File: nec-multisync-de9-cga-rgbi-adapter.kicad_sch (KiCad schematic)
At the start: 8 parts, among them J1 DE9_Plug, J2 DE15_Receptacle_HighDensity, J3 DIN-8

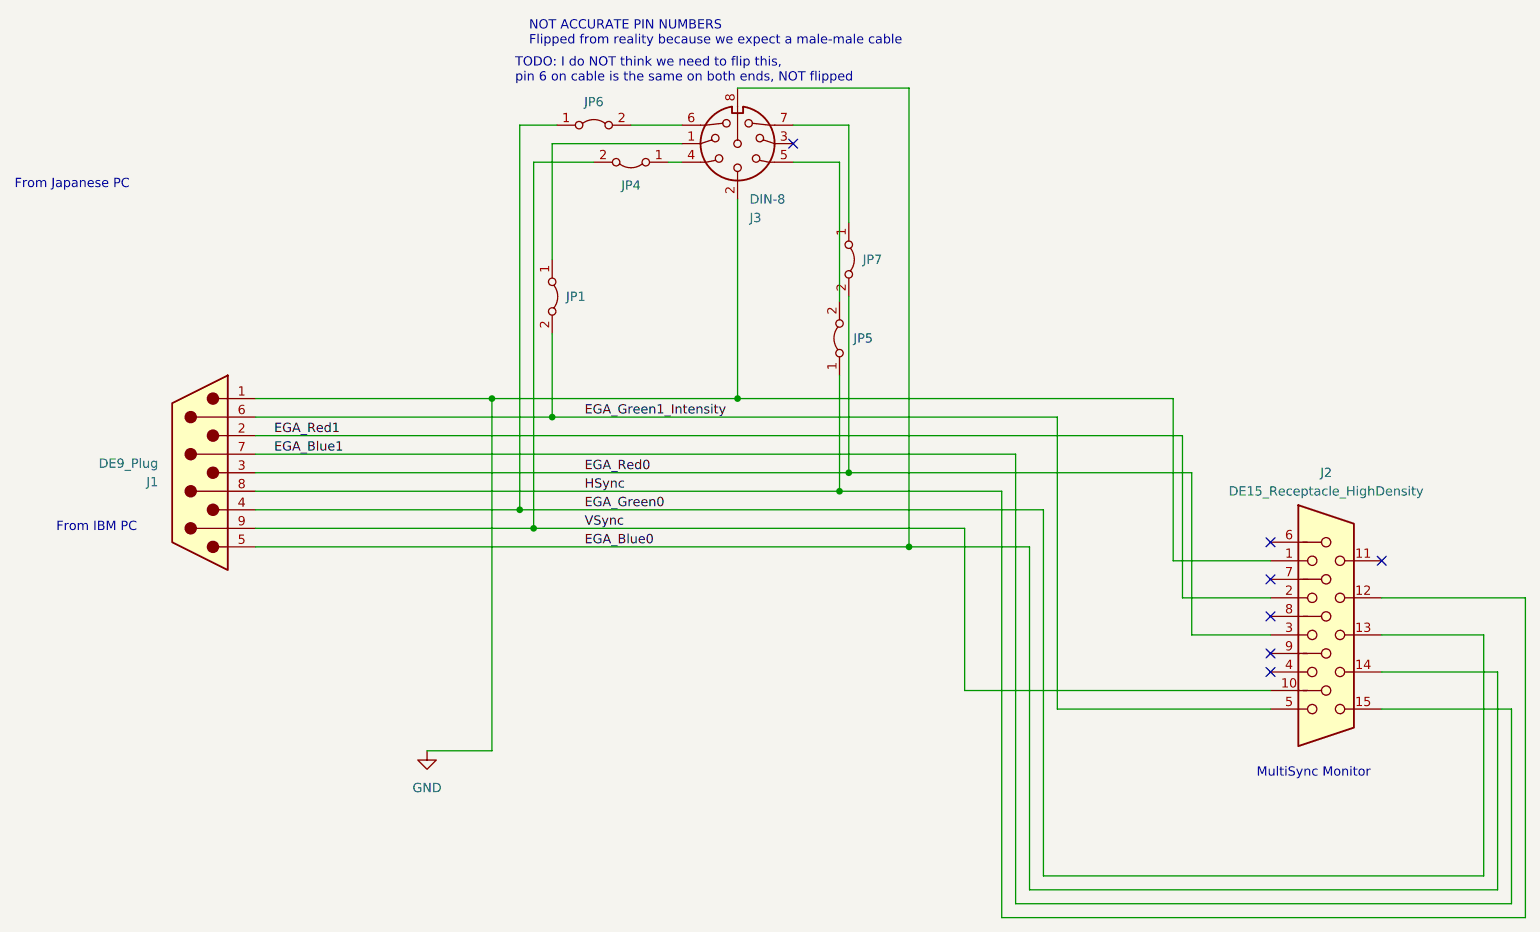
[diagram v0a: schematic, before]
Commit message: World's ugliest reroute
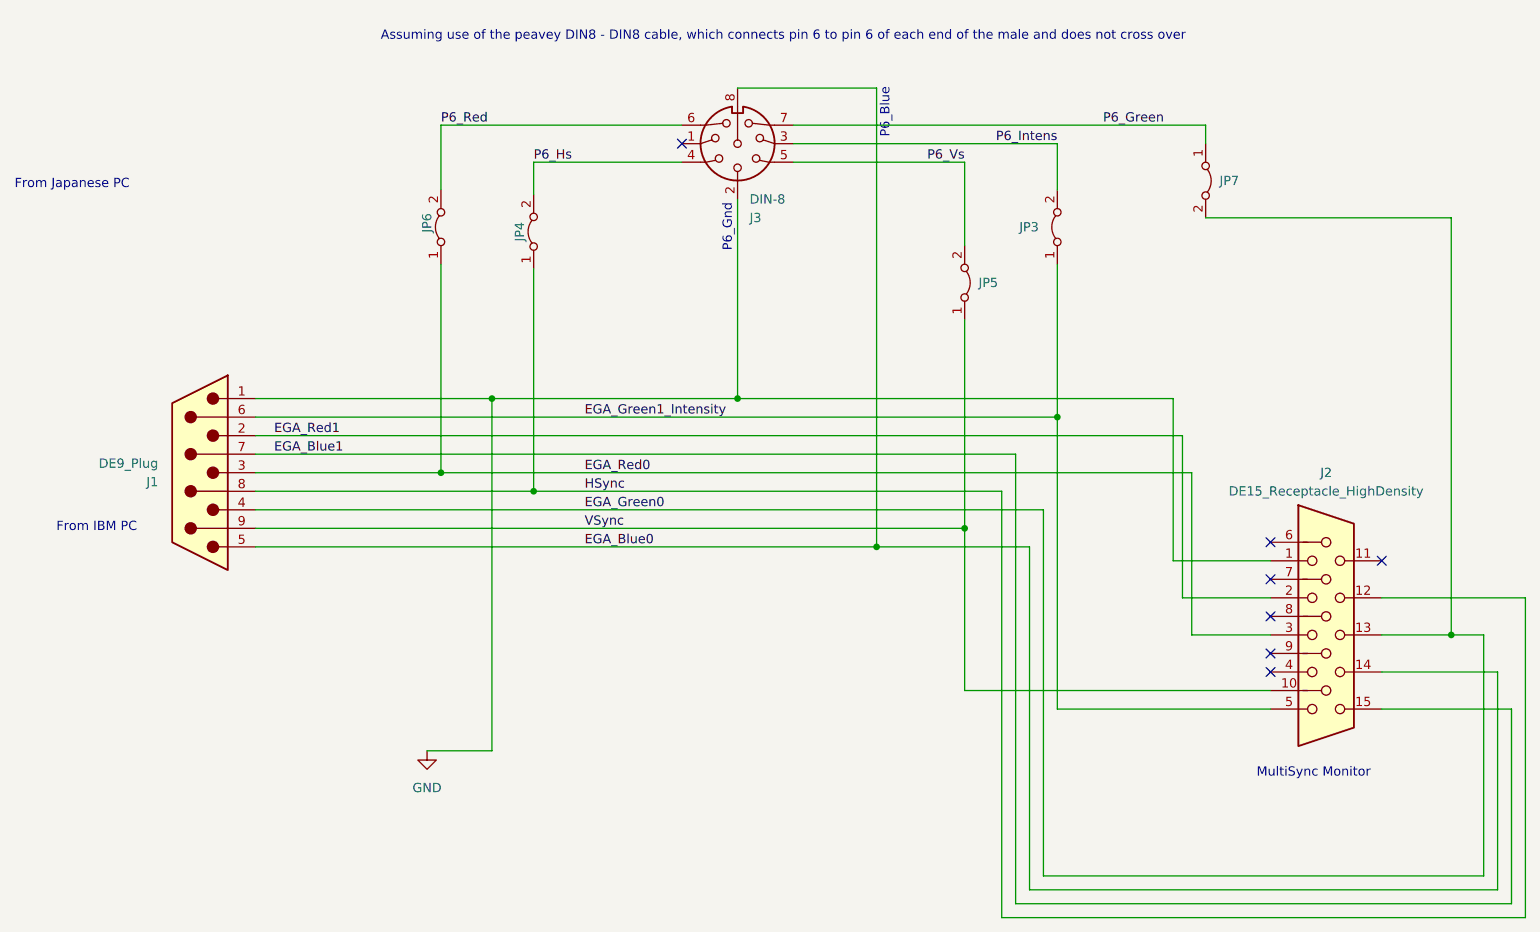
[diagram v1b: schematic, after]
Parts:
- renumbered JP1 to JP3
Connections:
- net EGA_Green0: now also JP7.2 (B); no longer JP6.1 (A)
- net EGA_Green1_Intensity: now also JP3.1 (A); no longer JP3.2 (B)
- net EGA_Red0: now also JP6.1 (A); no longer JP7.2 (B)
- net HSync: now also JP4.1 (A); no longer JP5.1 (A)
- net VSync: now also JP5.1 (A); no longer JP4.2 (B)
- net P6_Vs: now reaches J3.5, JP5.2 (B)
- net P6_Red: now reaches J3.6, JP6.2 (B)
- net P6_Green: now reaches J3.7, JP7.1 (A)
- net at J3.1: no longer JP3.1 (A)
- net P6_Intens: now reaches J3.3
- net P6_Intens: now also JP3.2 (B)
- net P6_Hs: now reaches J3.4
- net P6_Hs: now also JP4.2 (B); no longer JP4.1 (A)
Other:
- note added: "Assuming use of the peavey DIN8 - DIN8 cable, which connects pin 6 to pin 6 of each end of the male and does not cross over"
- note added: "P6_Blue"
- note added: "P6_Gnd"
- note removed: "NOT ACCURATE PIN NUMBERS Flipped from reality because we expect a male-male cable"
- note removed: "TODO: I do NOT think we need to flip this, pin 6 on cable is the same on both ends, NOT flipped"
- moved on the sheet: JP3, JP4, JP5, JP6, JP7
